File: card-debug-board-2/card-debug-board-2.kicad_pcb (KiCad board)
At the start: 2 copper layers, 36.9 x 55 mm, 33 parts, among them J1 2-1734592-0, J2 Conn_01x05, J5 0676430910, J6 629105150521, SW1 PCM13SMTR, SW2 B3F-1000, SW5 210-2LPS, U1 MIC5205-3.3YM5

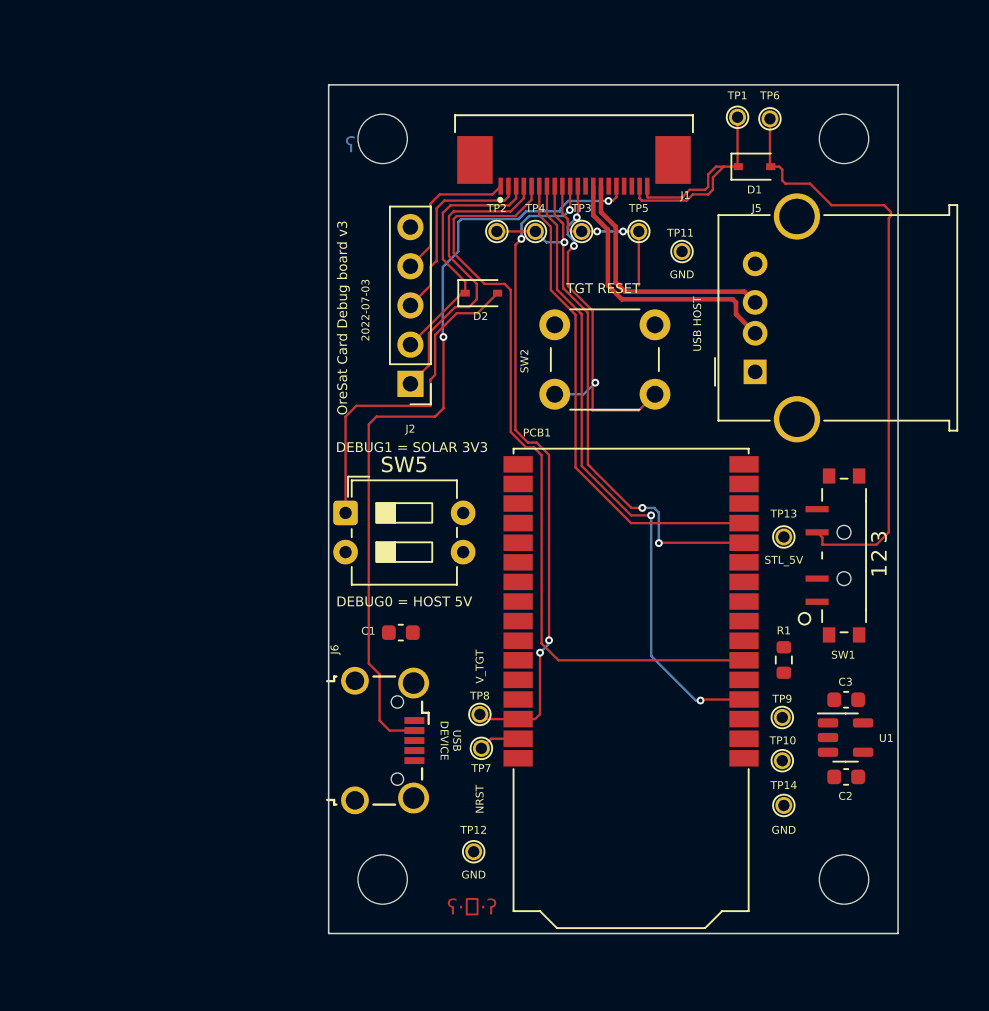
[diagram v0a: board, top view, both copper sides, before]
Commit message: Debug Board V3
DONE(??????)
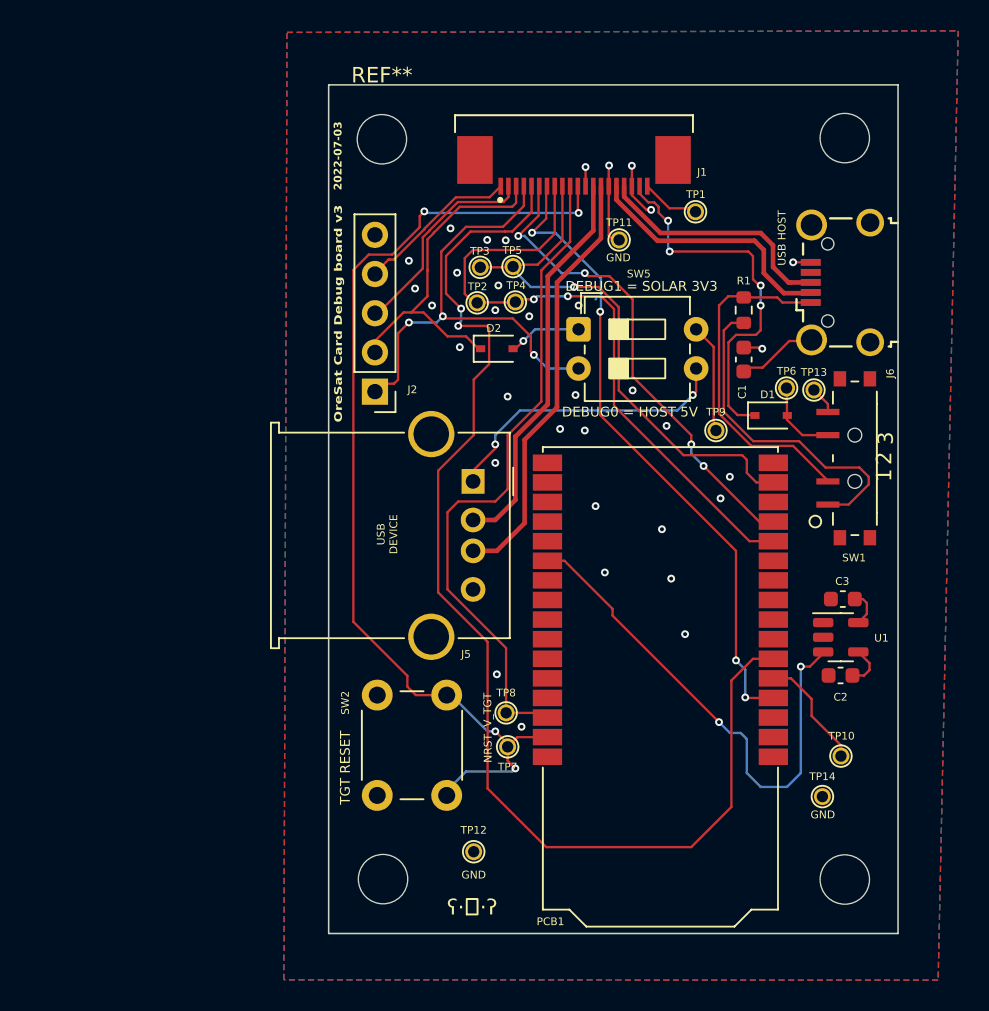
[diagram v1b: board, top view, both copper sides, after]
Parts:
- removed the REF** at (176.5, 50.0)
- removed the REF** at (146.6, 98.0)
- removed the REF** at (176.5, 98.0)
- removed the REF** at (146.6, 50.0)
- added REF**: MountingHole_3.2mm_M3, MountingHole:MountingHole_3.2mm_M3, F.Cu at (176.6, 98.0)
- added REF**: MountingHole_3.2mm_M3, MountingHole:MountingHole_3.2mm_M3, F.Cu at (146.6, 98.0)
- added REF**: MountingHole_3.2mm_M3, MountingHole:MountingHole_3.2mm_M3, F.Cu at (176.6, 50.0)
- added REF**: MountingHole_3.2mm_M3, MountingHole:MountingHole_3.2mm_M3, F.Cu at (146.6, 50.0)
- moved J6 41.8 mm to (176.2, 59.3), turned to 90 degrees
- moved SW2 32.6 mm to (146.2, 92.5), turned to 90 degrees
- moved C1 28.4 mm to (170.0, 64.3), turned to 90 degrees
- moved R1 22.8 mm to (170.0, 61.1)
- moved J5 19.6 mm to (152.5, 72.2), turned to -90 degrees
- moved SW5 19.2 mm to (159.3, 62.3)
- moved TP9 19.1 mm to (168.2, 68.9)
- moved TP6 17.5 mm to (172.8, 66.2)
- moved D1 16.2 mm to (171.8, 67.9)
- moved TP13 9.72 mm to (174.6, 66.3)
- moved TP5 8.46 mm to (155.1, 58.3)
- moved TP3 6.97 mm to (152.9, 58.3)
- moved TP1 6.70 mm to (166.9, 54.7)
- moved C2 6.58 mm to (176.3, 84.8)
- moved C3 6.53 mm to (176.4, 79.8)
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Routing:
- net Net-(J1-NRST): track 26.0 -> 64.7 mm, vias 3 -> 4
- net +5V: track 0.00 -> 35.1 mm, vias 0 -> 2
- net Net-(J1-DEVICE-D-): track 51.6 -> 16.9 mm, vias 2 -> 0
- net Net-(D1-A): track 38.9 -> 5.11 mm
- net Net-(J1-SWO): track 50.9 -> 77.9 mm, vias 0 -> 2
- net Net-(J1-CARD-RX): track 10.9 -> 36.2 mm, vias 2 -> 1
- net Net-(J6-VBUS): track 0.00 -> 22.2 mm
- net Net-(R1-Pad2): track 0.00 -> 21.6 mm
- net Net-(J5-VBUS): track 0.00 -> 18.7 mm, vias 0 -> 2
- net Net-(D2-A): track 21.9 -> 4.77 mm, vias 0 -> 1
- net Net-(J1-DEVICE-D+): track 0.00 -> 15.9 mm
- net GND: track 0.00 -> 12.7 mm, vias 0 -> 34
- net Net-(J1-HOST-D+): track 16.2 -> 28.0 mm
- net /DEBUG0/5VUSBHOST: track 20.0 -> 30.3 mm, vias 0 -> 3
- net Net-(D1-K): track 18.8 -> 28.4 mm, vias 0 -> 4
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- added copper zone on B.Cu, net GND
- added copper zone on F.Cu, net GND
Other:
- board text removed: "STL_5V"

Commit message: restore v2 card debug board files
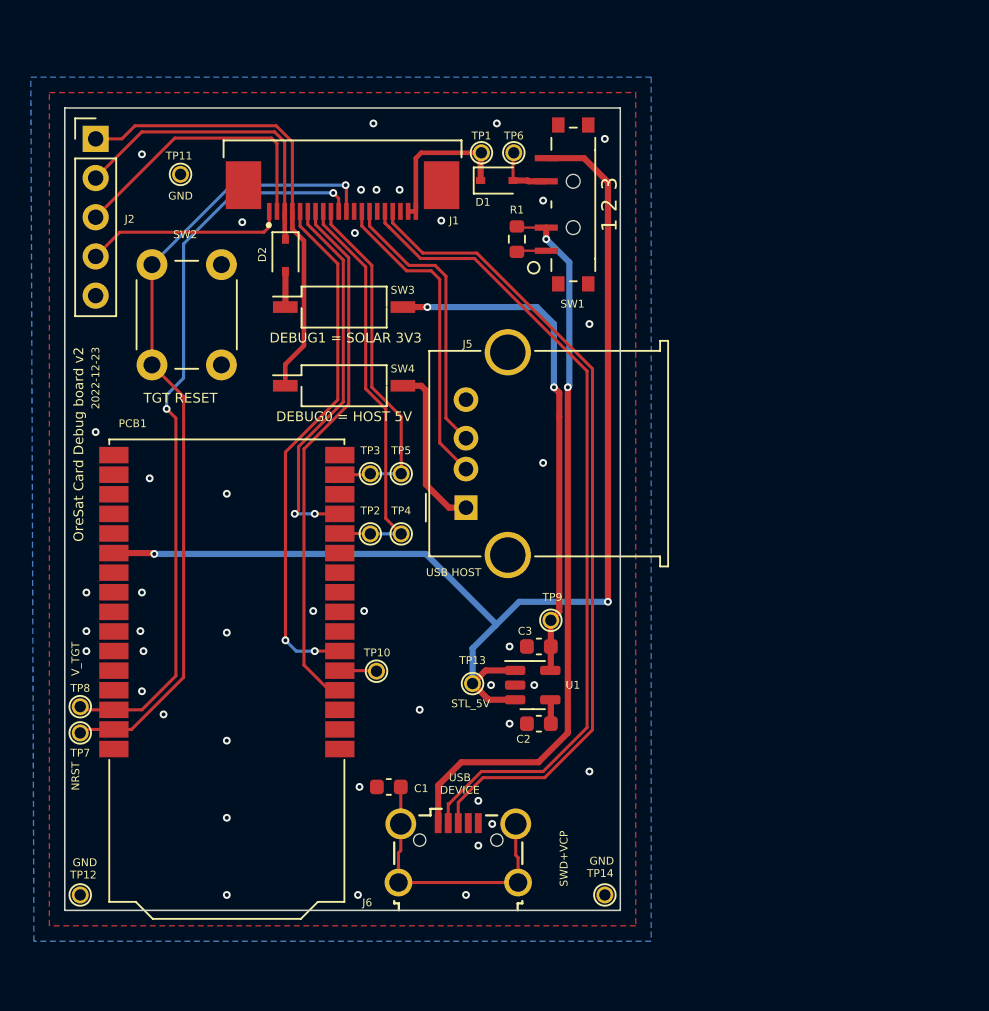
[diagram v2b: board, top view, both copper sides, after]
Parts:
- removed REF** (x4): MountingHole_3.2mm_M3, MountingHole:MountingHole_3.2mm_M3
- removed SW5: 210-2LPS, Button_Switch_THT:SW_DIP_SPSTx02_Slide_6.7x6.64mm_W7.62mm_P2.54mm_LowProfile
- added SW3: CFS-0103TB, Button_Switch_SMD:SW_DIP_SPSTx01_Slide_Copal_CHS-01B_W7.62mm_P1.27mm, F.Cu at (144.1, 60.9)
- added SW4: CFS-0103TB, Button_Switch_SMD:SW_DIP_SPSTx01_Slide_Copal_CHS-01B_W7.62mm_P1.27mm, F.Cu at (144.1, 66.0)
- J1: value 2-1734592-0 -> 2-1734592-0
- moved J6 44.5 mm to (151.5, 96.2), turned to 0 degrees
- moved C1 36.0 mm to (147.0, 92.0), turned to 180 degrees
- moved SW2 35.9 mm to (136.2, 58.1), turned to -90 degrees
- moved TP10 30.6 mm to (146.2, 84.5)
- moved TP13 29.2 mm to (152.4, 85.3)
- moved TP11 28.7 mm to (133.5, 52.3)
- moved PCB1 28.1 mm to (136.5, 99.5)
- moved TP7 27.7 mm to (127.0, 88.5)
- moved TP8 27.6 mm to (127.0, 86.8)
- moved TP12 25.7 mm to (127.0, 99.0)
- moved SW1 24.6 mm to (158.9, 54.2)
- moved J2 24.4 mm to (128.0, 50.0), turned to 0 degrees
- moved D1 23.4 mm to (154.0, 52.7)
- moved TP6 23.3 mm to (155.1, 50.9)
- moved U1 20.2 mm to (156.3, 85.4)
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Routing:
- net Net-(J1-SWO): track 77.9 -> 34.0 mm
- net +5V: track 35.1 -> 77.1 mm
- net Net-(J1-DEVICE-D+): track 15.9 -> 53.0 mm
- net Net-(J1-DEVICE-D-): track 16.9 -> 53.2 mm
- net Net-(J6-VBUS): track 22.2 -> 47.6 mm, vias 0 -> 2
- net +3.3V: track 9.47 -> 33.1 mm, vias 0 -> 2
- net Net-(R1-Pad2): track 21.6 -> 1.94 mm
- net Net-(D1-K): track 28.4 -> 10.2 mm, vias 4 -> 0
- net Net-(J1-CARD-TX): track 42.6 -> 27.0 mm, vias 2 -> 0
- net Net-(J1-CARD-RX): track 36.2 -> 22.9 mm, vias 1 -> 0
- net GND: track 12.7 -> 0.00 mm, vias 34 -> 42
- net Net-(J6-Shield): track 5.36 -> 17.9 mm
- net Net-(J1-NRST): track 64.7 -> 52.2 mm, vias 4 -> 1
- net Net-(J1-HOST-D+): track 28.0 -> 18.3 mm
- net Net-(J5-VBUS): track 18.7 -> 10.9 mm, vias 2 -> 0
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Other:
- board size 36.9 x 55 mm -> 36 x 52 mm
- board text added: "2022-12-23"
- board text added: "OreSat Card Debug board v2"
- board text added: "STL_5V"
- board text added: "SWD+VCP"
- board text removed: "2022-07-03"
- board text removed: "OreSat Card Debug board v3"
- board text removed: "ʕ·ᴥ·ʔ﻿"
